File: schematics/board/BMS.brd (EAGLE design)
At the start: 68 x 22 mm, 11 parts

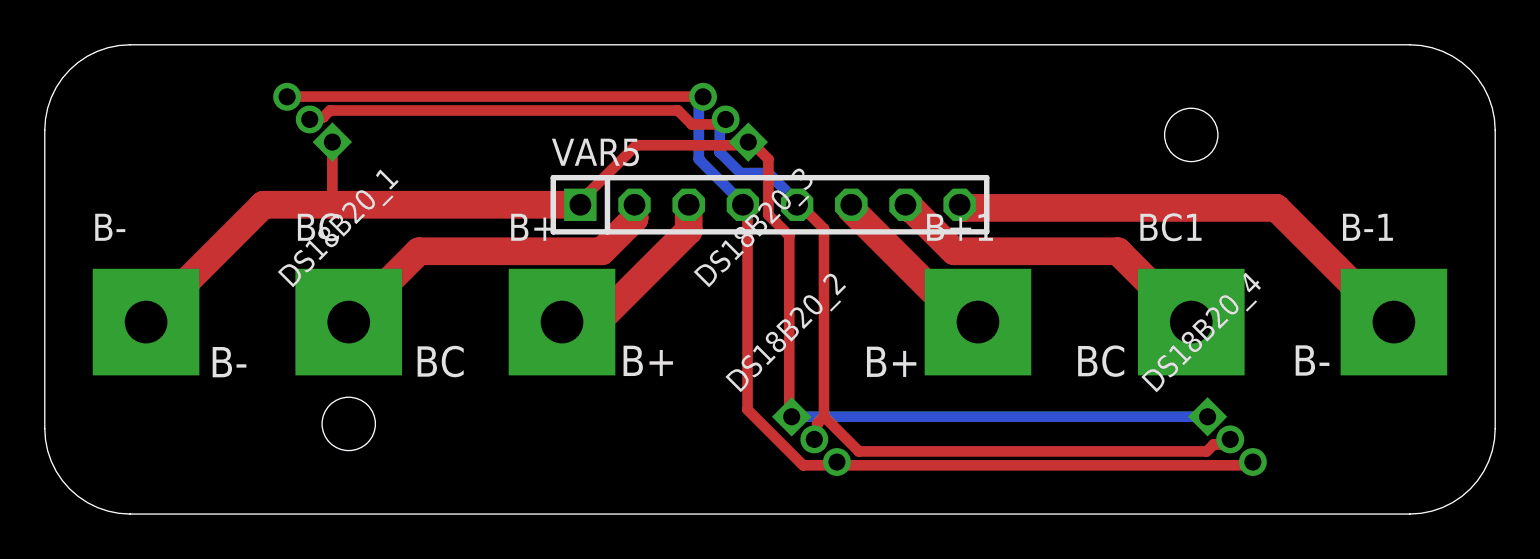
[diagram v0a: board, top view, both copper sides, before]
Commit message: Новые схемы
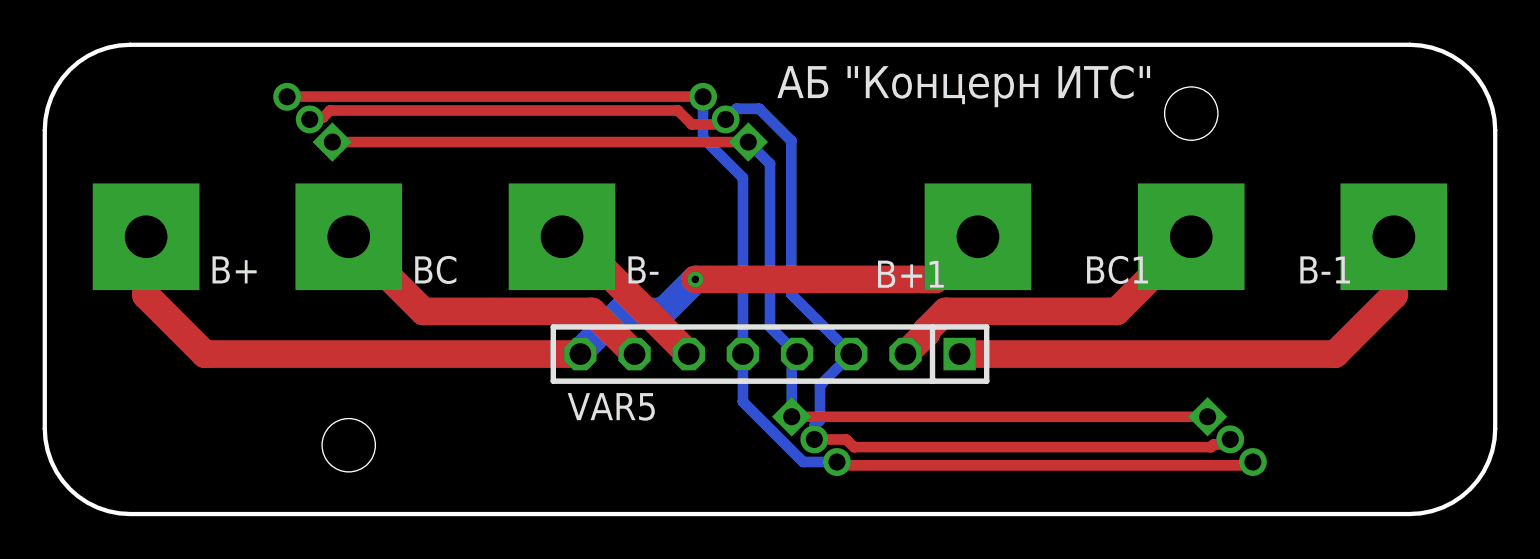
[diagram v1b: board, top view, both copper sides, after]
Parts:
- moved B+ 19.9 mm to (4.75, 13.0)
- moved B- 19.9 mm to (24.2, 13.0)
- moved VAR5 7.00 mm to (34.0, 7.50), turned to 180 degrees
- moved B+1 4.00 mm to (43.8, 13.0)
- moved B-1 4.00 mm to (63.2, 13.0)
- moved BC 4.00 mm to (14.2, 13.0)
- moved BC1 4.00 mm to (53.8, 13.0)
- renumbered DS18B20_1 to DS18B20B, DS18B20_2 to DS18B20A, DS18B20_3 to DS18B20, DS18B20_4 to DS18B20C
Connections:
- removed net B-5: B+.P$44, VAR5.3
- removed net GND: B-.P$44, DS18B20.1, DS18B20A.1, DS18B20B.1, DS18B20C.1, VAR5.1
- new net N$1: DS18B20.1, DS18B20A.1, DS18B20B.1, DS18B20C.1, VAR5.4
- new net N$2: B-.P$44, VAR5.6
- net 1W: now also VAR5.3; no longer VAR5.5
- net BMS+: now also B+.P$44, VAR5.8; no longer VAR5.6
- net N$205: now also VAR5.7; no longer VAR5.2
- net N$206: now also VAR5.2; no longer VAR5.7
- net N$3: now also VAR5.1; no longer VAR5.8
- net VDD: now also VAR5.5; no longer VAR5.4
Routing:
- net GND: track 68.2 -> 0.00 mm
- net N$1: track 0.00 -> 52.9 mm
- net BMS+: track 8.34 -> 45.2 mm, vias 0 -> 1
- net B-5: track 8.93 -> 0.00 mm
- net N$2: track 0.00 -> 8.22 mm
- net N$3: track 22.6 -> 24.2 mm
- net 1W: track 58.2 -> 59.6 mm
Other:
- board text added: "АБ "Концерн ИТС""
- board text removed: "B+"
- board text removed: "B-"
- board text removed: "BC"
